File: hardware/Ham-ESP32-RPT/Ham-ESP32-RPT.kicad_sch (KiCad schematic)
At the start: 19 parts, among them J1 USB_C_Receptacle_USB2.0_16P, J2 Conn_Coaxial, U1 ESP32-S3-WROOM-1, U2 D3V3XA4B10LP, U3 TLV75801PDBV, U4 ESP32-S3-DevKitC

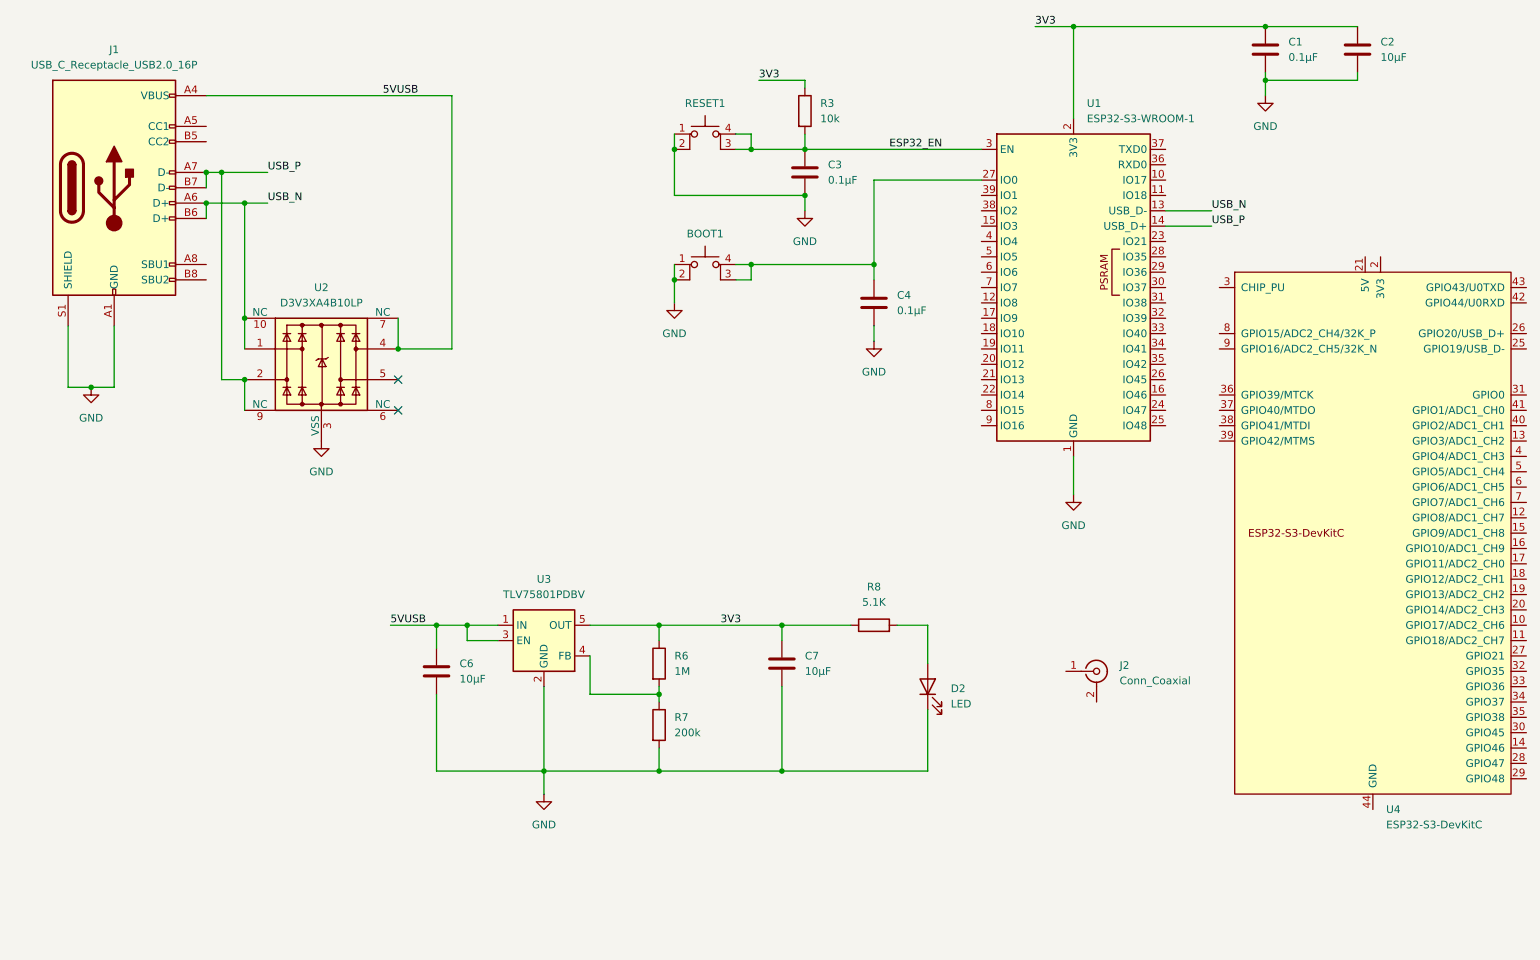
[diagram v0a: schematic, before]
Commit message: doc HAM-ESP32
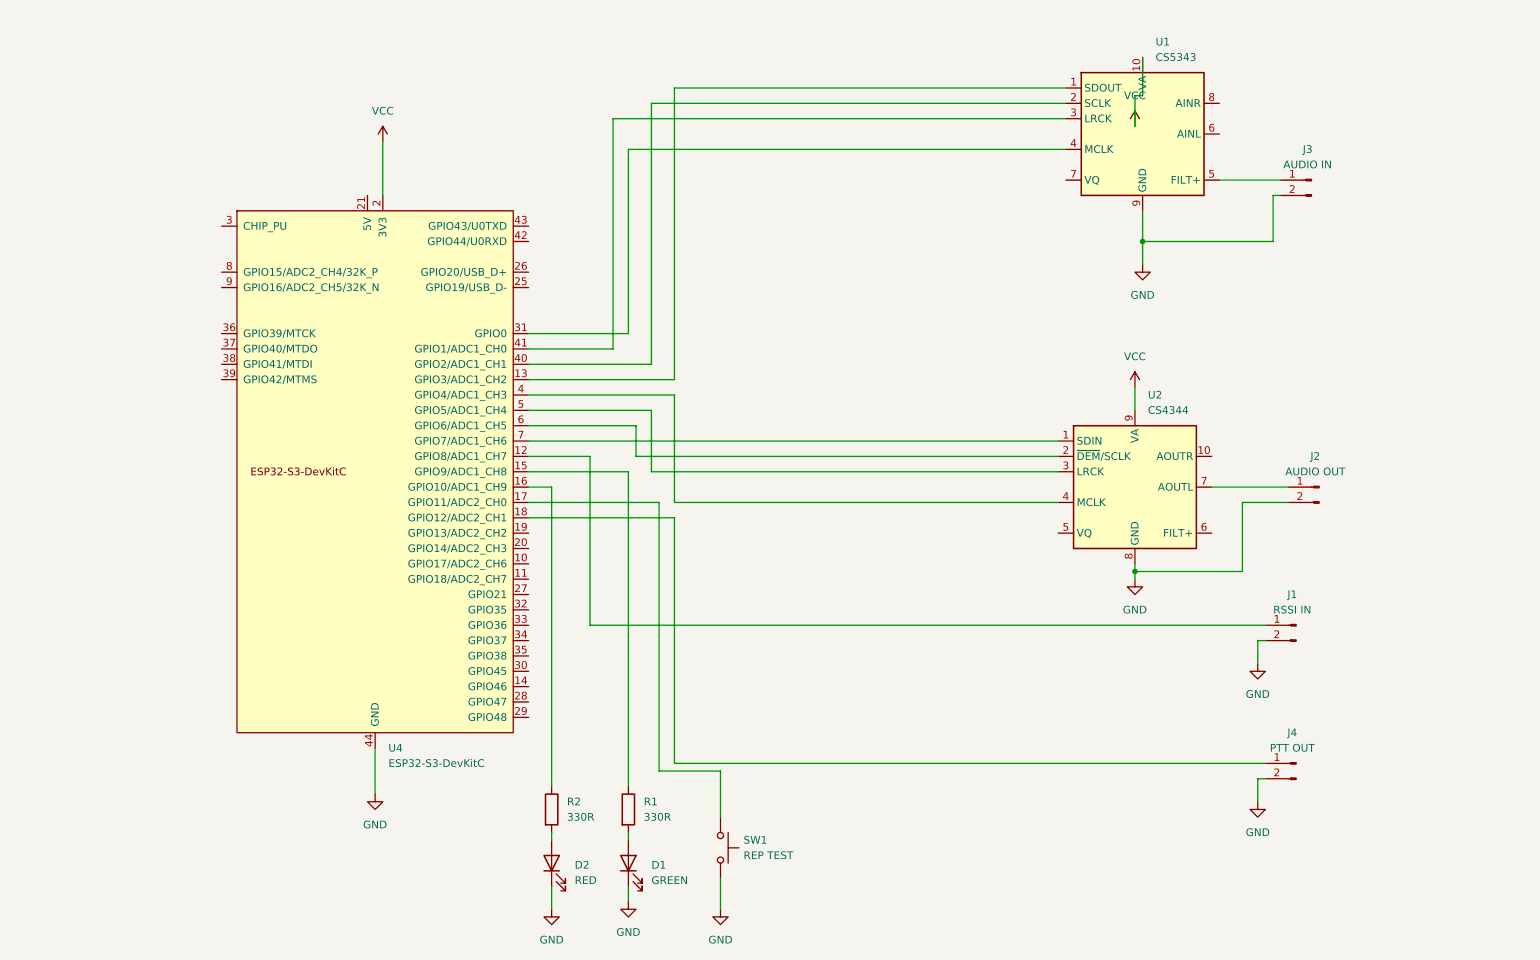
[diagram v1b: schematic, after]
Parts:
- removed BOOT1, RESET1: SW_MEC_5E, Button_Switch_SMD:SW_MEC_5GSH9, symbol PCM_Switch:SW_MEC_5E
- removed C1, C3, C4: 0.1µF, Capacitor_SMD:C_0805_2012Metric, symbol Device:C
- removed C2, C6, C7: 10µF, Capacitor_SMD:C_0805_2012Metric, symbol Device:C
- removed J1: USB_C_Receptacle_USB2.0_16P, Connector_USB:USB_C_Receptacle_GCT_USB4085, symbol Connector:USB_C_Receptacle_USB2.0_16P
- removed J2: Conn_Coaxial, Connector_Coaxial:SMA_Molex_73251-1153_EdgeMount_Horizontal, symbol Connector:Conn_Coaxial
- removed R3: 10k, Resistor_SMD:R_0805_2012Metric, symbol Device:R
- removed R6: 1M, Resistor_SMD:R_0805_2012Metric, symbol Device:R
- removed R7: 200k, Resistor_SMD:R_0805_2012Metric, symbol Device:R
- removed R8: 5.1K, Resistor_SMD:R_0805_2012Metric, symbol Device:R
- removed U1: ESP32-S3-WROOM-1, RF_Module:ESP32-S3-WROOM-1U, symbol RF_Module:ESP32-S3-WROOM-1
- removed U2: D3V3XA4B10LP, Package_DFN_QFN:Diodes_UDFN-10_1.0x2.5mm_P0.5mm, symbol Power_Protection:D3V3XA4B10LP
- removed U3: TLV75801PDBV, Package_TO_SOT_SMD:SOT-23-5, symbol Regulator_Linear:TLV75801PDBV
- added D1: GREEN, symbol Device:LED
- added J1: RSSI IN, symbol Connector:Conn_01x02_Pin
- added J2: AUDIO OUT, symbol Connector:Conn_01x02_Pin
- added J3: AUDIO IN, symbol Connector:Conn_01x02_Pin
- added J4: PTT OUT, symbol Connector:Conn_01x02_Pin
- added R1, R2: 330R, symbol Device:R
- added SW1: REP TEST, symbol Switch:SW_Push
- added U1: CS5343, Package_SO:TSSOP-10_3x3mm_P0.5mm, symbol Audio:CS5343
- added U2: CS4344, Package_SO:TSSOP-10_3x3mm_P0.5mm, symbol Audio:CS4344
- D2: value LED -> RED; footprint LED_SMD:LED_0805_2012Metric -> (none)
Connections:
- net GND: now also U4.22 (GND), U4.23 (GND), U4.24 (GND), U4.44 (GND), D1.1 (K), J1.2 (Pin_2), J2.2 (Pin_2), J3.2 (Pin_2), J4.2 (Pin_2), SW1.2, U1.9 (GND), U2.8 (GND)
- net at D2.2 (A): now also R2.2
- net VCC: now reaches U4.1 (3V3), U4.2 (3V3)
- net VCC: now also U1.10 (VA), U2.9 (VA)
- net at U4.12 (GPIO8/ADC1_CH7): now also J1.1 (Pin_1)
- net at U4.13 (GPIO3/ADC1_CH2): now also U1.1 (SDOUT)
- net at U4.15 (GPIO9/ADC1_CH8): now also R1.1
- net at U4.16 (GPIO10/ADC1_CH9): now also R2.1
- net at U4.17 (GPIO11/ADC2_CH0): now also SW1.1
- net at U4.18 (GPIO12/ADC2_CH1): now also J4.1 (Pin_1)
- net at U4.31 (GPIO0): now also U1.4 (MCLK)
- net at U4.4 (GPIO4/ADC1_CH3): now also U2.4 (MCLK)
- net at U4.40 (GPIO2/ADC1_CH1): now also U1.2 (SCLK)
- net at U4.41 (GPIO1/ADC1_CH0): now also U1.3 (LRCK)
- net at U4.5 (GPIO5/ADC1_CH4): now also U2.3 (LRCK)
- net at U4.6 (GPIO6/ADC1_CH5): now also U2.2 (~{DEM}/SCLK)
- net at U4.7 (GPIO7/ADC1_CH6): now also U2.1 (SDIN)
- new net: J3.1 (Pin_1), U1.5 (FILT+)
- new net: J2.1 (Pin_1), U2.7 (AOUTL)
- new net: D1.2 (A), R1.2
- no-connect marks 2 -> 0
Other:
- moved on the sheet: U4
